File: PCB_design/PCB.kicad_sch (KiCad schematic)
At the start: 3 parts, among them U1 BME280, U2 SeeeduinoXIAO

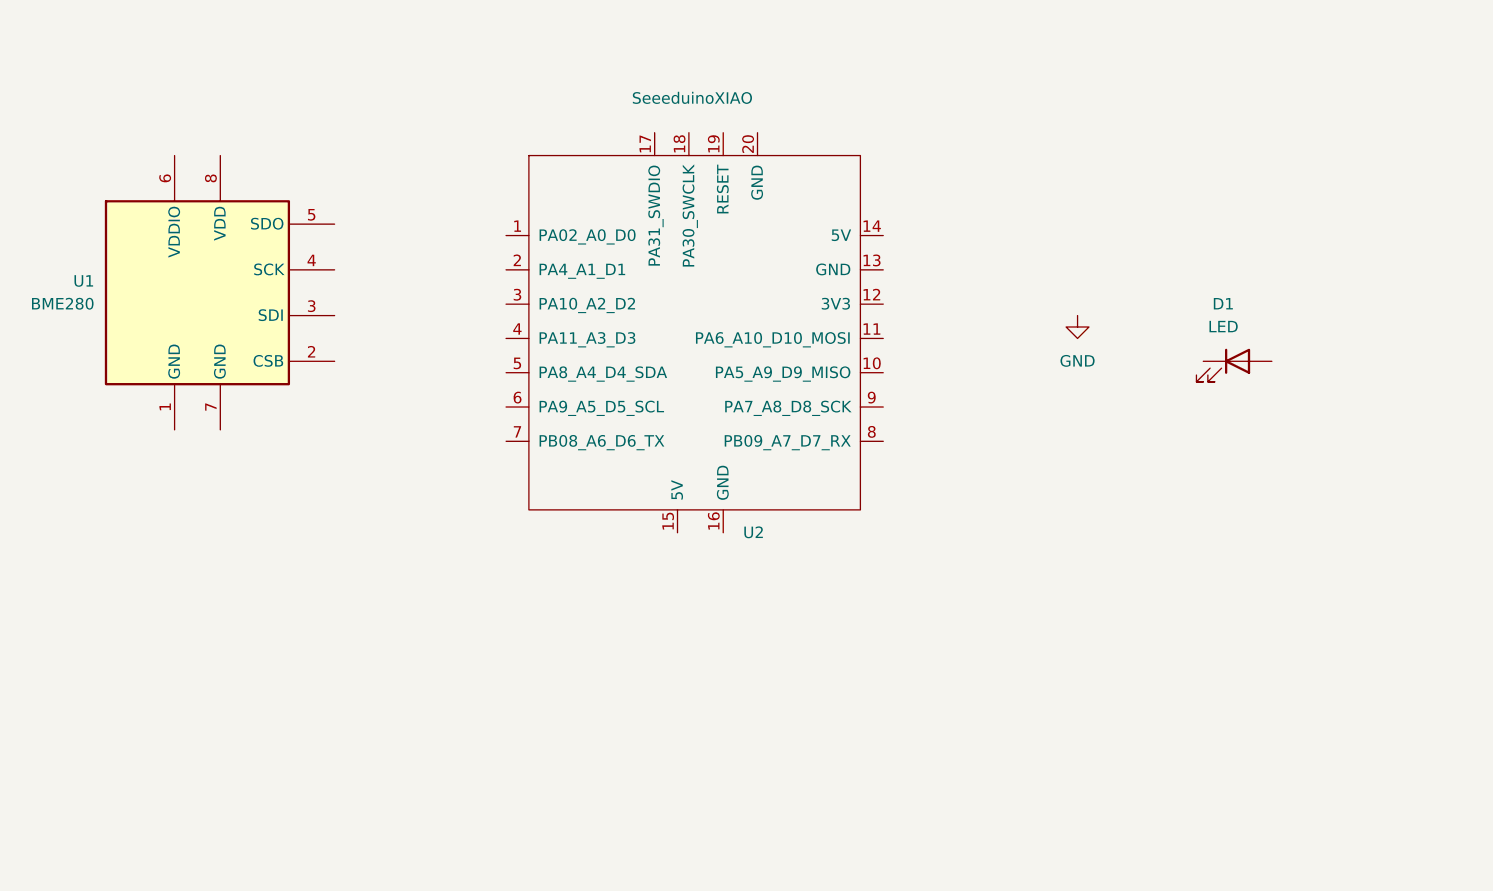
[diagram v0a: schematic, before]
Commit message: MODIFY README.md
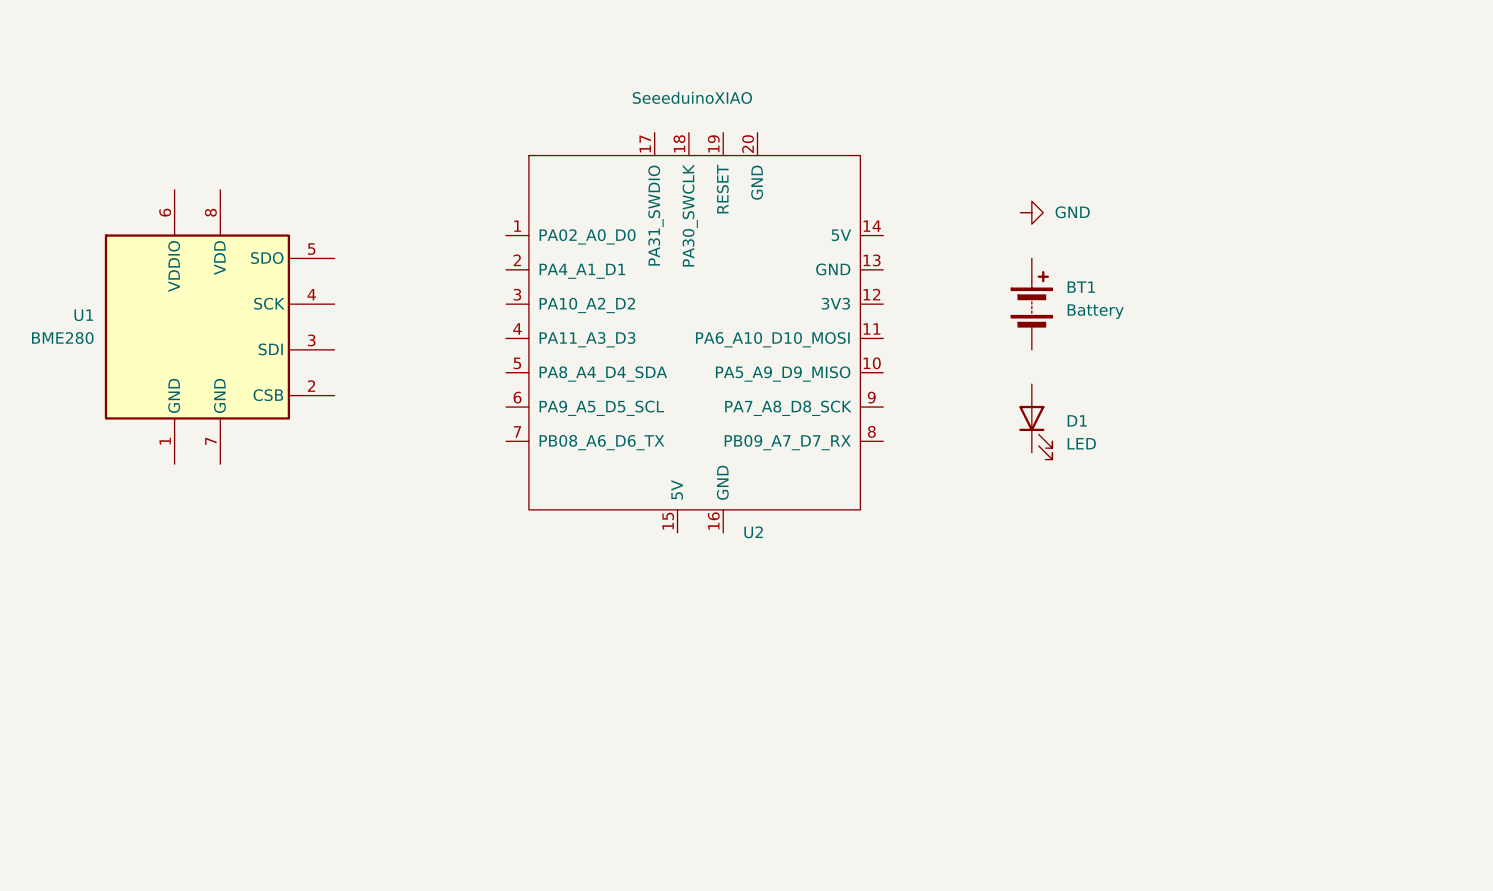
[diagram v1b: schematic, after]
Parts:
- added BT1: Battery, symbol Device:Battery
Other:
- moved on the sheet: D1, U1
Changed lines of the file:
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@@
 (kicad_sch (version 20230121) (generator eeschema)
   (paper "A4")
-  (symbol (lib_id "Device:LED") (at 231.14 87.63 0) (unit 1)
+  (symbol (lib_id "Device:LED") (at 208.28 93.98 90) (unit 1)
     (in_bom yes) (on_board yes) (dnp no) (fields_autoplaced)
-    (property "Reference" "D1" (at 229.5525 81.28 0)
-      (effects (font (size 1.27 1.27)))
+    (property "Reference" "D1" (at 212.09 94.2975 90)
+      (effects (font (size 1.27 1.27)) (justify right))
     )
-    (property "Value" "LED" (at 229.5525 83.82 0)
-      (effects (font (size 1.27 1.27)))
+    (property "Value" "LED" (at 212.09 96.8375 90)
+      (effects (font (size 1.27 1.27)) (justify right))
     )
-    (property "Footprint" "" (at 231.14 87.63 0)
+    (property "Footprint" "" (at 208.28 93.98 0)
       (effects (font (size 1.27 1.27)) hide)
     )
-    (property "Datasheet" "~" (at 231.14 87.63 0)
+    (property "Datasheet" "~" (at 208.28 93.98 0)
       (effects (font (size 1.27 1.27)) hide)
     )
@@
     )
   )
-  (symbol (lib_id "Sensor:BME280") (at 115.57 80.01 0) (unit 1)
+  (symbol (lib_id "Sensor:BME280") (at 115.57 83.82 0) (unit 1)
     (in_bom yes) (on_board yes) (dnp no) (fields_autoplaced)
-    (property "Reference" "U1" (at 104.14 78.74 0)
+    (property "Reference" "U1" (at 104.14 82.55 0)
       (effects (font (size 1.27 1.27)) (justify right))
     )
-    (property "Value" "BME280" (at 104.14 81.28 0)
+    (property "Value" "BME280" (at 104.14 85.09 0)
       (effects (font (size 1.27 1.27)) (justify right))
     )
-    (property "Footprint" "Package_LGA:Bosch_LGA-8_2.5x2.5mm_P0.65mm_ClockwisePinNumbering" (at 153.67 91.44 0)
+    (property "Footprint" "Package_LGA:Bosch_LGA-8_2.5x2.5mm_P0.65mm_ClockwisePinNumbering" (at 153.67 95.25 0)
       (effects (font (size 1.27 1.27)) hide)
     )
-    (property "Datasheet" "https://www.bosch-sensortec.com/media/boschsensortec/downloads/datasheets/bst-bme280-ds002.pdf" (at 115.57 85.09 0)
+    (property "Datasheet" "https://www.bosch-sensortec.com/media/boschsensortec/downloads/datasheets/bst-bme280-ds002.pdf" (at 115.57 88.9 0)
       (effects (font (size 1.27 1.27)) hide)
     )
@@
         (path "/79b0a8cb-7144-418a-acde-3d2f1fae0f6b"
           (reference "U1") (unit 1)
+        )
+      )
+    )
+  )
+  (symbol (lib_id "Device:Battery") (at 208.28 81.28 0) (unit 1)
+    (in_bom yes) (on_board yes) (dnp no) (fields_autoplaced)
+    (property "Reference" "BT1" (at 212.09 79.4385 0)
+      (effects (font (size 1.27 1.27)) (justify left))
+    )
+    (property "Value" "Battery" (at 212.09 81.9785 0)
+      (effects (font (size 1.27 1.27)) (justify left))
+    )
+    (property "Footprint" "" (at 208.28 79.756 90)
+      (effects (font (size 1.27 1.27)) hide)
+    )
+    (property "Datasheet" "~" (at 208.28 79.756 90)
+      (effects (font (size 1.27 1.27)) hide)
+    )
+    (pin "1")
+    (pin "2")
+    (instances
+      (project "PCB"
+        (path "/79b0a8cb-7144-418a-acde-3d2f1fae0f6b"
+          (reference "BT1") (unit 1)
         )
       )
@@
     )
   )
-  (symbol (lib_id "power:GND") (at 213.36 82.55 0) (unit 1)
+  (symbol (lib_id "power:GND") (at 207.01 71.12 90) (unit 1)
     (in_bom yes) (on_board yes) (dnp no) (fields_autoplaced)
-    (property "Reference" "#PWR01" (at 213.36 88.9 0)
+    (property "Reference" "#PWR01" (at 213.36 71.12 0)
       (effects (font (size 1.27 1.27)) hide)
     )
-    (property "Value" "GND" (at 213.36 87.63 0)
-      (effects (font (size 1.27 1.27)))
+    (property "Value" "GND" (at 210.82 71.12 90)
+      (effects (font (size 1.27 1.27)) (justify right))
     )
-    (property "Footprint" "" (at 213.36 82.55 0)
+    (property "Footprint" "" (at 207.01 71.12 0)
       (effects (font (size 1.27 1.27)) hide)
     )
-    (property "Datasheet" "" (at 213.36 82.55 0)
+    (property "Datasheet" "" (at 207.01 71.12 0)
       (effects (font (size 1.27 1.27)) hide)
     )

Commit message: update datasheet
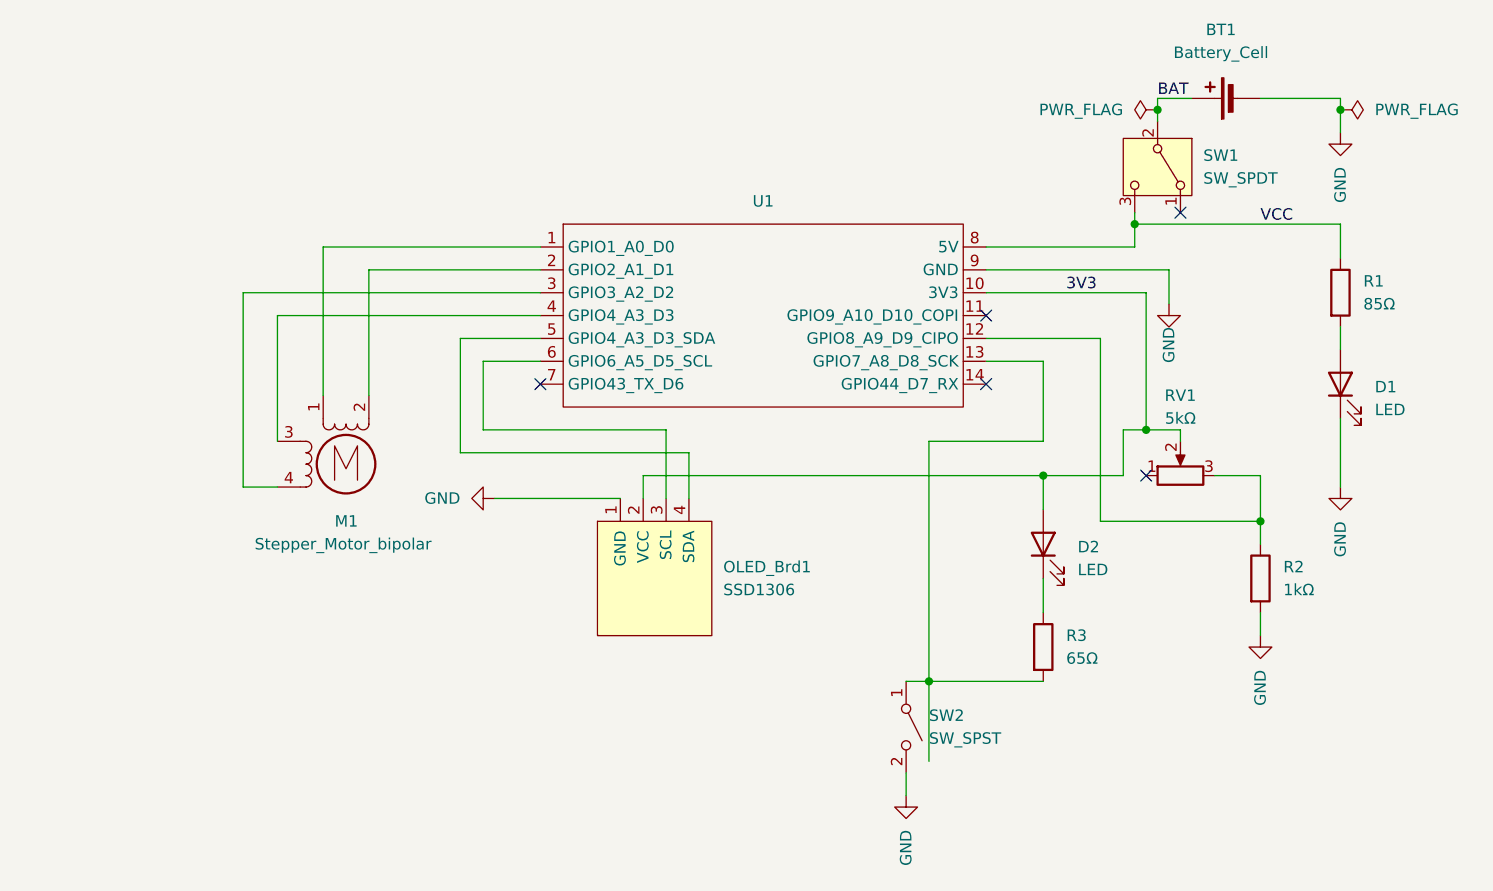
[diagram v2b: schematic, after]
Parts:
- removed BT1: Battery, symbol Device:Battery
- removed U1: BME280, Package_LGA:Bosch_LGA-8_2.5x2.5mm_P0.65mm_ClockwisePinNumbering, symbol Sensor:BME280
- removed U2: SeeeduinoXIAO, Seeeduino-XIAO:Seeeduino XIAO-MOUDLE14P-2.54-21X17.8MM, symbol Seeeduino-XIAO:SeeeduinoXIAO
- added BT1: Battery_Cell, Connector_JST:JST_NV_B02P-NV_1x02_P5.00mm_Vertical, symbol Device:Battery_Cell
- added D2: LED, LED_SMD:LED_0805_2012Metric_Pad1.15x1.40mm_HandSolder, symbol Device:LED
- added M1: Stepper_Motor_bipolar, demo motor:x27_stepper, symbol Motor:Stepper_Motor_bipolar
- added OLED_Brd1: SSD1306, demo ssd1306:128x64OLED, symbol ssd1306_oled:SSD1306
- added R1: 85Ω, Resistor_SMD:R_0805_2012Metric_Pad1.20x1.40mm_HandSolder, symbol Device:R
- added R2: 1kΩ, Resistor_SMD:R_0805_2012Metric_Pad1.20x1.40mm_HandSolder, symbol Device:R
- added R3: 65Ω, Resistor_SMD:R_0805_2012Metric_Pad1.20x1.40mm_HandSolder, symbol Device:R
- added RV1: 5kΩ, Potentiometer_THT:Potentiometer_Piher_PC-16_Single_Horizontal, symbol Device:R_Potentiometer
- added SW1: SW_SPDT, Connector_JST:JST_EH_B3B-EH-A_1x03_P2.50mm_Vertical, symbol Switch:SW_SPDT
- added SW2: SW_SPST, Button_Switch_THT:SW_PUSH-12mm, symbol Switch:SW_SPST
- added U1: ~, demo xiao:XIAO_ESP32_SENSE, symbol seeeduino xiao esp32:XIAO_ESP32_SENSE
- D1: footprint (none) -> LED_SMD:LED_0805_2012Metric_Pad1.15x1.40mm_HandSolder
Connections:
- net GND: now also D1.1 (K), BT1.2 (-), OLED_Brd1.1 (GND), R2.2, SW2.2 (B), U1.9 (GND)
- net at D1.2 (A): now also R1.2
- new net: R2.1, RV1.3, U1.12 (GPIO8_A9_D9_CIPO)
- new net: D2.1 (K), R3.1
- new net: M1.1, U1.1 (GPIO1_A0_D0)
- new net: M1.2 (-), U1.2 (GPIO2_A1_D1)
- new net: M1.3, U1.4 (GPIO4_A3_D3)
- new net: M1.4, U1.3 (GPIO3_A2_D2)
- new net: OLED_Brd1.3 (SCL), U1.6 (GPIO6_A5_D5_SCL)
- new net: OLED_Brd1.4 (SDA), U1.5 (GPIO4_A3_D3_SDA)
- new net: R3.2, SW2.1 (A), U1.13 (GPIO7_A8_D8_SCK)
- new net 3V3: D2.2 (A), OLED_Brd1.2 (VCC), RV1.2, U1.10 (3V3)
- new net BAT: BT1.1 (+), SW1.2 (B)
- new net VCC: R1.1, SW1.3 (C), U1.8 (5V)
- no-connect marks 0 -> 5
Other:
- company: (none) -> Chelsey Lee
- title: (none) -> PCB_Controller
- moved on the sheet: D1
